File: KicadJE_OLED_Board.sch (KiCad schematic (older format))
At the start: 43 parts, among them J101 Out1, J102 IN1, J103 OUT1, J104 OutFlt, J105 INFLT, J106 OUTFLT, J107 In1, J108 InFlt, P101 Doepfer_Power_10pin, U101 TL072

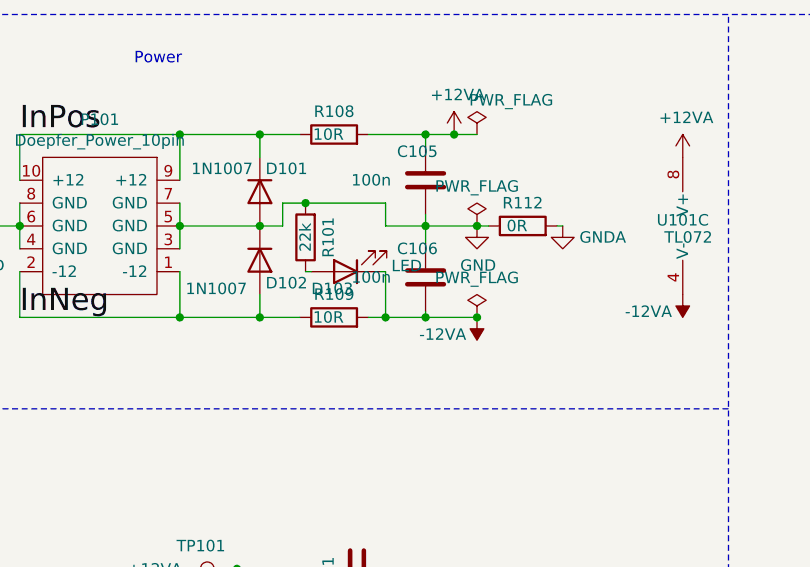
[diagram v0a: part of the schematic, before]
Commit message: placed amp/filt
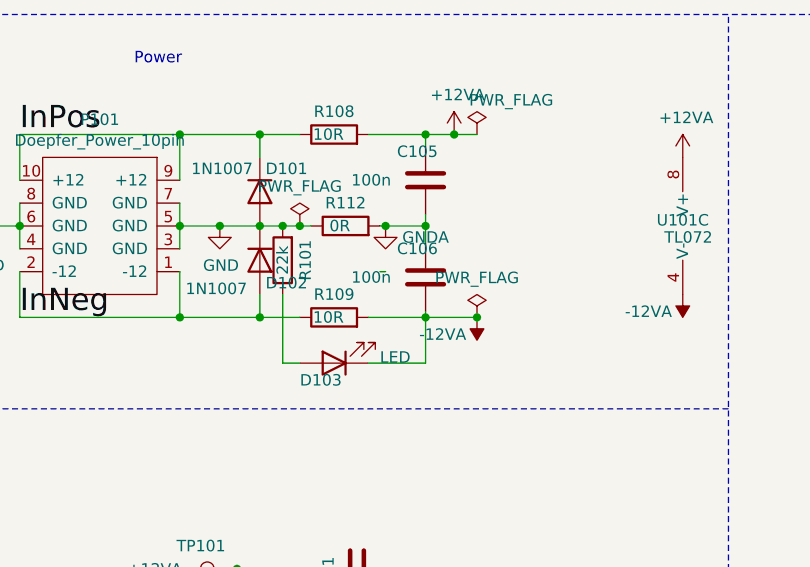
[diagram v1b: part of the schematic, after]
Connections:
- net GND: no longer C105.2, C106.1
- net GNDA: now also C105.2, C106.1
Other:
- moved on the sheet: D103, R101, R112
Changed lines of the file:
@@
 L power:PWR_FLAG #FLG?
 U 1 1 5F4F8A4F
-P 3400 1450
+P 2625 1450
 AR Path="/5E4B0DD9/5F4F8A4F" Ref="#FLG?"  Part="1"
 AR Path="/5E62ACA1/5F4F8A4F" Ref="#FLG?"  Part="1"
 AR Path="/5F49A670/5F4F8A4F" Ref="#FLG?"  Part="1"
 AR Path="/5F4F8A4F" Ref="#FLG0102"  Part="1"
-F 0 "#FLG0102" H 3400 1525 50  0001 C CNN
-F 1 "PWR_FLAG" H 3400 1623 50  0000 C CNN
-F 2 "" H 3400 1450 50  0001 C CNN
-F 3 "~" H 3400 1450 50  0001 C CNN
-	1    3400 1450
+F 0 "#FLG0102" H 2625 1525 50  0001 C CNN
+F 1 "PWR_FLAG" H 2625 1623 50  0000 C CNN
+F 2 "" H 2625 1450 50  0001 C CNN
+F 3 "~" H 2625 1450 50  0001 C CNN
+	1    2625 1450
 	1    0    0    -1
 $EndComp
@@
 L Device:R R101
 U 1 1 5F4F8A6F
-P 2650 1500
+P 2550 1600
 AR Path="/5F4F8A6F" Ref="R101"  Part="1"
 AR Path="/5C8C5FC0/5F4F8A6F" Ref="R?"  Part="1"
@@
 AR Path="/5E62ACA1/5F4F8A6F" Ref="R?"  Part="1"
 AR Path="/5F49A670/5F4F8A6F" Ref="R?"  Part="1"
-F 0 "R101" V 2550 1500 50  0000 C CNN
-F 1 "22k" V 2650 1500 50  0000 C CNN
-F 2 "AJ:R_0805_AJ" V 2580 1500 50  0001 C CNN
-F 3 "~" H 2650 1500 50  0001 C CNN
-	1    2650 1500
+F 0 "R101" V 2450 1600 50  0000 C CNN
+F 1 "22k" V 2550 1600 50  0000 C CNN
+F 2 "AJ:R_0805_AJ" V 2480 1600 50  0001 C CNN
+F 3 "~" H 2550 1600 50  0001 C CNN
+	1    2550 1600
 	-1   0    0    1
 $EndComp
-Connection ~ 3400 1450
+Connection ~ 2625 1450
 Connection ~ 3400 1850
 $Comp
@@
 L Device:LED D?
 U 1 1 5F4F8ACC
-P 2825 1650
+P 2775 2050
 AR Path="/5E4B0DD9/5F4F8ACC" Ref="D?"  Part="1"
 AR Path="/5E62ACA1/5F4F8ACC" Ref="D?"  Part="1"
 AR Path="/5F49A670/5F4F8ACC" Ref="D?"  Part="1"
 AR Path="/5F4F8ACC" Ref="D103"  Part="1"
-F 0 "D103" H 2975 1725 50  0000 R CNN
-F 1 "LED" H 2625 1625 50  0000 R CNN
-F 2 "AJ:D_0805_AJ" H 2825 1650 50  0001 C CNN
-F 3 "~" H 2825 1650 50  0001 C CNN
-	1    2825 1650
+F 0 "D103" H 2925 2125 50  0000 R CNN
+F 1 "LED" H 2575 2025 50  0000 R CNN
+F 2 "AJ:D_0805_AJ" H 2775 2050 50  0001 C CNN
+F 3 "~" H 2775 2050 50  0001 C CNN
+	1    2775 2050
 	-1   0    0    1
 $EndComp
@@
 $EndComp
 Wire Wire Line
-	3000 1650 3000 1850
-Connection ~ 3000 1850
-Wire Wire Line
 	2450 1750 2450 1850
 Wire Wire Line
@@
 	3000 1650 2975 1650
 Wire Wire Line
-	2650 1650 2675 1650
-Wire Wire Line
-	3000 1350 2650 1350
-Wire Wire Line
-	2650 1350 2550 1350
-Wire Wire Line
-	2550 1350 2550 1450
-Wire Wire Line
 	2550 1450 2450 1450
-Connection ~ 2650 1350
 Wire Notes Line
 	525  525  525  7725
@@
 Wire Wire Line
 	2450 1050 2625 1050
-Wire Wire Line
-	3000 1450 3000 1350
 $Comp
 L power:GND #PWR0102
 U 1 1 6074CFAE
-P 3400 1450
-F 0 "#PWR0102" H 3400 1200 50  0001 C CNN
-F 1 "GND" H 3405 1277 50  0000 C CNN
-F 2 "" H 3400 1450 50  0001 C CNN
-F 3 "" H 3400 1450 50  0001 C CNN
-	1    3400 1450
+P 2275 1450
+F 0 "#PWR0102" H 2275 1200 50  0001 C CNN
+F 1 "GND" H 2280 1277 50  0000 C CNN
+F 2 "" H 2275 1450 50  0001 C CNN
+F 3 "" H 2275 1450 50  0001 C CNN
+	1    2275 1450
 	1    0    0    -1
 $EndComp
 Wire Wire Line
 	3000 1450 3175 1450
-Wire Wire Line
-	3000 1850 3175 1850
 Wire Wire Line
 	2450 1850 2625 1850
@@
 L power:GNDA #PWR0145
 U 1 1 6226F578
-P 3775 1450
+P 3000 1450
 AR Path="/6226F578" Ref="#PWR0145"  Part="1"
 AR Path="/5CD3F059/6226F578" Ref="#PWR?"  Part="1"
 AR Path="/608CA457/6226F578" Ref="#PWR?"  Part="1"
-F 0 "#PWR0145" H 3775 1200 50  0001 C CNN
-F 1 "GNDA" H 3950 1400 50  0000 C CNN
-F 2 "" H 3775 1450 50  0001 C CNN
-F 3 "" H 3775 1450 50  0001 C CNN
-	1    3775 1450
+F 0 "#PWR0145" H 3000 1200 50  0001 C CNN
+F 1 "GNDA" H 3175 1400 50  0000 C CNN
+F 2 "" H 3000 1450 50  0001 C CNN
+F 3 "" H 3000 1450 50  0001 C CNN
+	1    3000 1450
 	1    0    0    -1
 $EndComp
@@
 L Device:R R112
 U 1 1 6226FF55
-P 3600 1450
+P 2825 1450
 AR Path="/6226FF55" Ref="R112"  Part="1"
 AR Path="/5CD3F059/6226FF55" Ref="R?"  Part="1"
 AR Path="/608CA457/6226FF55" Ref="R?"  Part="1"
-F 0 "R112" V 3700 1450 50  0000 C CNN
-F 1 "0R" V 3600 1475 50  0000 C CNN
-F 2 "AJ:R_0805_AJ" V 3530 1450 50  0001 C CNN
-F 3 "~" H 3600 1450 50  0001 C CNN
-	1    3600 1450
-	0    -1   -1   0
-$EndComp
-Wire Wire Line
-	3400 1450 3450 1450
-Wire Wire Line
-	3750 1450 3775 1450
+F 0 "R112" V 2925 1450 50  0000 C CNN
+F 1 "0R" V 2825 1475 50  0000 C CNN
+F 2 "AJ:R_0805_AJ" V 2755 1450 50  0001 C CNN
+F 3 "~" H 2825 1450 50  0001 C CNN
+	1    2825 1450
+	0    -1   -1   0
+$EndComp
+Wire Wire Line
+	2625 1450 2675 1450
+Wire Wire Line
+	2975 1450 3000 1450
 $Comp
 L Eurorack:Doepfer_Power_10pin P101
@@
 	2100 1450 2100 1350
 Wire Wire Line
-	2450 1450 2100 1450
+	2450 1450 2275 1450
 Wire Wire Line
 	2450 1850 2100 1850
@@
 	0    -1   -1   0
 $EndComp
-Wire Wire Line
-	2925 1850 3000 1850
 $Comp
 L Amplifier_Operational:TL072 U?
@@
 Connection ~ 3175 1450
 Wire Wire Line
-	3175 1450 3400 1450
-Wire Wire Line
 	3175 1450 3175 1525
 Text Label 1400 1050 0    97   ~ 0
@@
 	1775 3425 1975 3425
 $Comp
-L power:GNDA #PWR?
+L power:GNDA #PWR0152
 U 1 1 623419A2
 P 1375 3650
-AR Path="/623419A2" Ref="#PWR?"  Part="1"
+AR Path="/623419A2" Ref="#PWR0152"  Part="1"
 AR Path="/5CD3F059/623419A2" Ref="#PWR?"  Part="1"
 AR Path="/608CA457/623419A2" Ref="#PWR?"  Part="1"
-F 0 "#PWR?" H 1375 3400 50  0001 C CNN
+F 0 "#PWR0152" H 1375 3400 50  0001 C CNN
 F 1 "GNDA" H 1550 3600 50  0000 C CNN
 F 2 "" H 1375 3650 50  0001 C CNN
@@
 P 5050 5325
 AR Path="/608CA457/6235C128" Ref="#PWR?"  Part="1"
-AR Path="/6235C128" Ref="#PWR?"  Part="1"
-F 0 "#PWR?" H 5050 5075 50  0001 C CNN
+AR Path="/6235C128" Ref="#PWR0153"  Part="1"
+F 0 "#PWR0153" H 5050 5075 50  0001 C CNN
 F 1 "GND" H 5055 5152 50  0000 C CNN
 F 2 "" H 5050 5325 50  0001 C CNN
@@
 	1    0    0    -1
 $EndComp
+Wire Wire Line
+	2925 1850 3175 1850
+Connection ~ 3000 1450
+Connection ~ 2275 1450
+Wire Wire Line
+	2275 1450 2100 1450
+Wire Wire Line
+	2550 1450 2625 1450
+Connection ~ 2550 1450
+Wire Wire Line
+	2550 1750 2550 2050
+Wire Wire Line
+	2550 2050 2625 2050
+Wire Wire Line
+	2925 2050 3175 2050
+Wire Wire Line
+	3175 2050 3175 1850
 $EndSCHEMATC
